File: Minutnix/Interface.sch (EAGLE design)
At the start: 15 parts

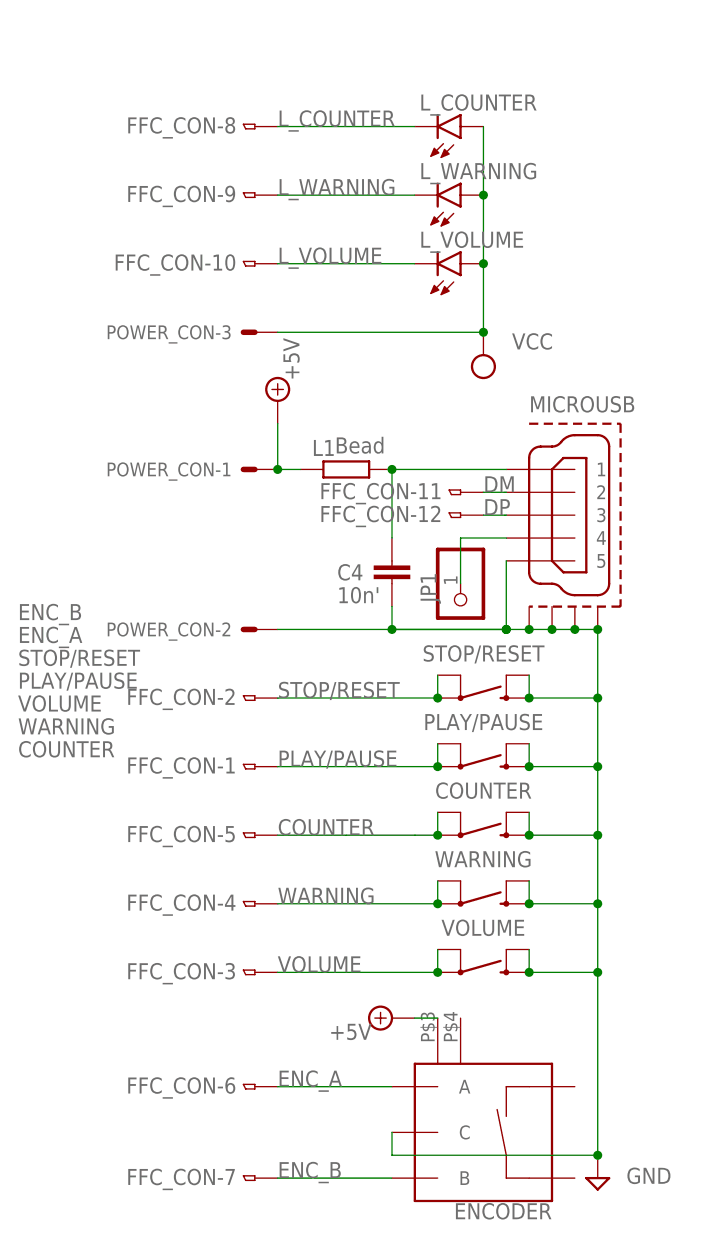
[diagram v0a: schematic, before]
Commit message: Final actualisation
Libs update
Change name from Ekspander to Interface
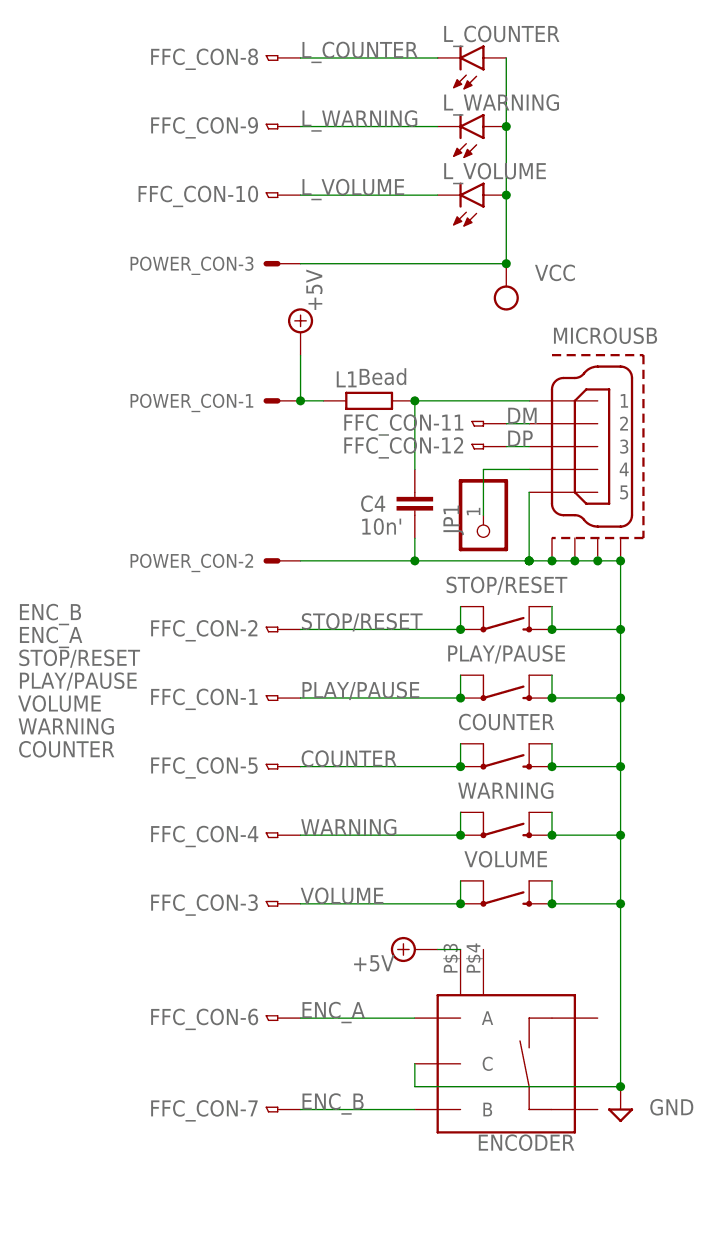
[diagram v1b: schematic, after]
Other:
- moved on the sheet: C4, COUNTER, ENCODER, FFC_CON-1, FFC_CON-10, FFC_CON-11, FFC_CON-12, FFC_CON-2, FFC_CON-3, FFC_CON-4, FFC_CON-5, FFC_CON-6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
